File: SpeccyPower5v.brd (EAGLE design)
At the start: 112.1 x 40 mm, 60 parts, among them T1 TRANS_ER29

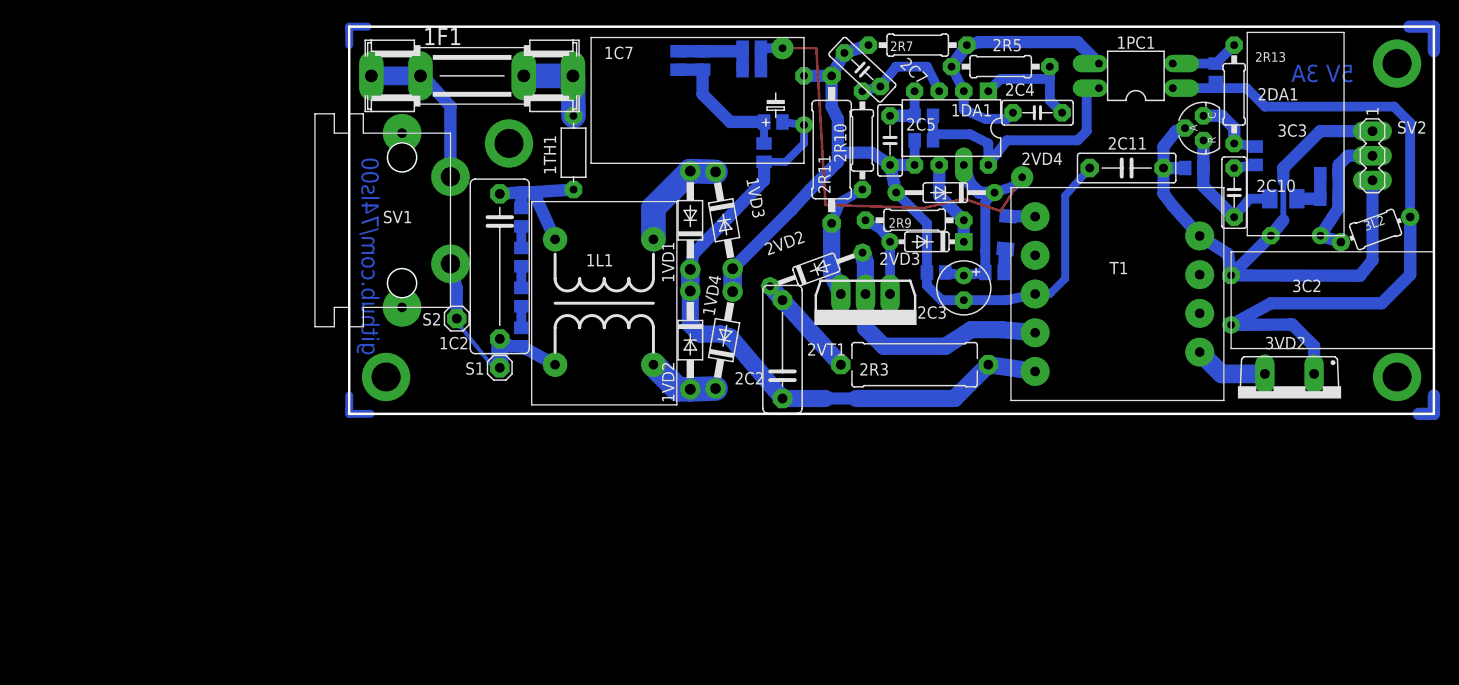
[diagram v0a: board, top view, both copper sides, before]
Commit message: test v h
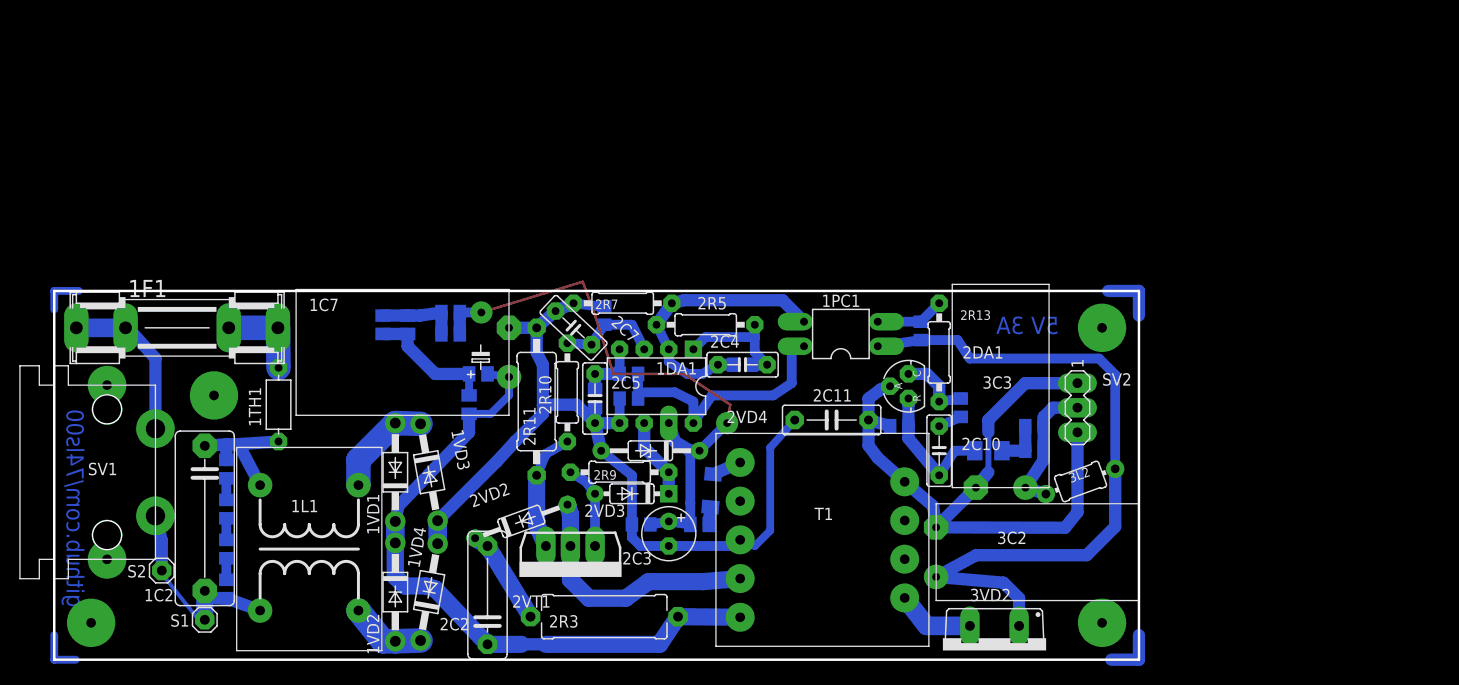
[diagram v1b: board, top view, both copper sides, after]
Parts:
- added 2C4A, 2C5A, 2C7A: (no value), rcl:C0805
- moved 2R1E 41.4 mm to (54.3, 68.6)
- moved 2R1F 41.4 mm to (54.3, 70.8)
- moved 2R3 41.3 mm to (70.2, 39.4)
- moved 2R1C 40.9 mm to (47.3, 69.5)
- moved 2R1D 40.9 mm to (49.8, 69.5)
- moved 2DA1 40.5 mm to (101.6, 63.2)
- moved 1DA1 40.5 mm to (75.6, 63.2)
- moved 1PC1 40.5 mm to (94.6, 68.6)
- moved 2C6 40.5 mm to (72.7, 61.9)
- moved 2R16 40.5 mm to (100.6, 59.1)
- moved 2R5 40.5 mm to (80.6, 69.5)
- moved 2R8 40.5 mm to (72.7, 64.5)
- moved 2VD1 40.5 mm to (81.3, 52.4)
- moved 2C10 40.5 mm to (104.8, 56.5)
- moved 2C5 40.5 mm to (69.2, 61.9)
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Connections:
- net N$23 renamed +IN
- removed net N$40: 1DA1.2, 1PC1.3, 2C4.2, 2R5.1, 2R7.2
- removed net N$6: 1DA1.1, 2C4.1, 2R5.2
- new net 817-3: 1DA1.2, 1PC1.3, 2C4.2, 2C4A.2, 2R5.1, 2R7.2
- new net COMP: 1DA1.1, 2C4.1, 2C4A.1, 2R5.2
- net -IN: now also 2C5A.2, 2C7A.2
- net N$3: now also 2C5A.1
- net N$4: now also 2C7A.1
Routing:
- net 817-3: track 0.00 -> 28.8 mm
- net N$40: track 27.6 -> 0.00 mm
- net COMP: track 0.00 -> 13.1 mm
- net N$6: track 12.2 -> 0.00 mm
- net +16IN: track 67.8 -> 61.7 mm
- net -IN: track 87.8 -> 92.0 mm
- net N$33: track 3.49 -> 5.40 mm
- net N$3: track 5.08 -> 6.67 mm
- net N$29: track 14.8 -> 13.6 mm
- net N$30: track 10.9 -> 10.1 mm
- net N$19: track 9.03 -> 8.28 mm
- net N$31: track 4.13 -> 4.76 mm
- net N$1: track 11.2 -> 10.6 mm
- net N$8: track 8.99 -> 8.35 mm
- net N$27: track 3.81 -> 4.45 mm
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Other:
- board size 112.1 x 40 mm -> 112.1 x 38.1 mm
